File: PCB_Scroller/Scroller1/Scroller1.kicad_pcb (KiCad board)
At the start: 2 copper layers, 154.8 x 94.6 mm, 66 parts

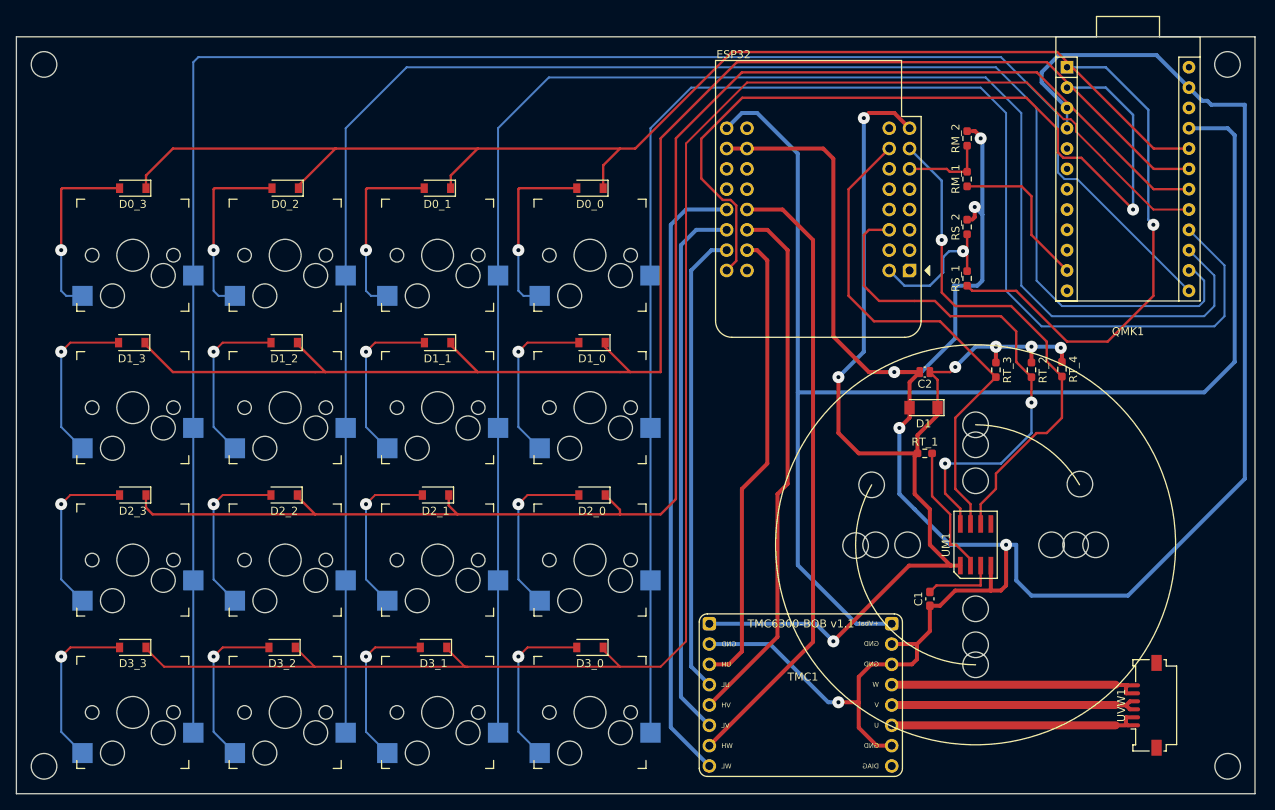
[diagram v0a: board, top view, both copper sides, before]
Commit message: Updates
Not sure if the ESP32 works...
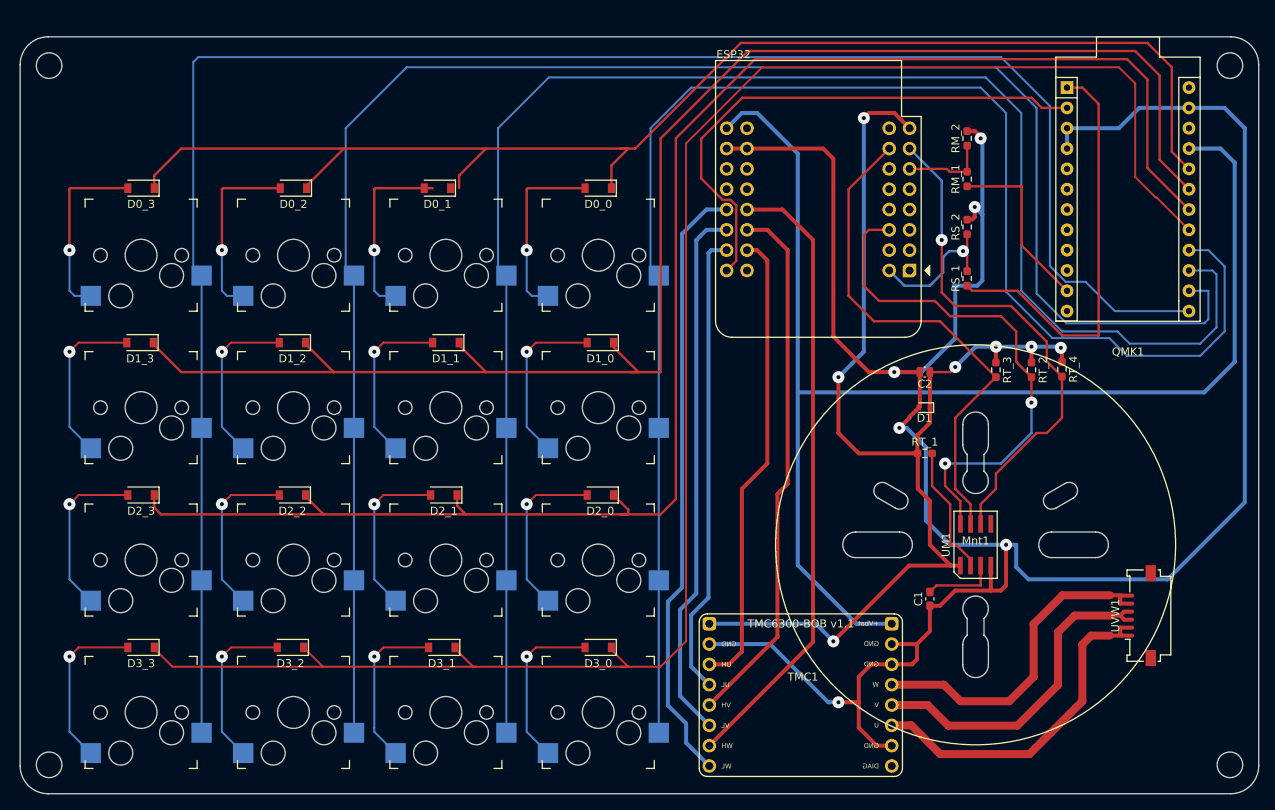
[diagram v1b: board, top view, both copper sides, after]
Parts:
- removed 2208_1, 2208_2, 2208_3, 2208_4, 3508_1, 3508_2, 3508_3, 3508_4, 6010_1, 6010_2, 6010_3, 6010_4, E6B2_1, E6B2_2: M3, MountingHole:MountingHole_3.2mm_M3
- added Mnt1: -, MT6701:BLDC Mount, F.Cu at (183.8, 117.1)
- D1: footprint Diode_SMD:D_MiniMELF -> Diode_SMD:D_SOD-523
- moved UVW1 11.2 mm to (203.9, 125.9)
- moved QMK1 2.54 mm to (210.4, 87.9)
- moved D0_0 1.04 mm to (136.6, 72.5)
- moved D0_2 1.04 mm to (98.5, 72.5)
- moved D1_0 1.04 mm to (136.8, 91.8)
- moved D1_2 1.04 mm to (98.4, 91.8)
- moved D1_3 1.04 mm to (79.3, 91.8)
- moved D2_0 1.04 mm to (136.8, 110.9)
- moved D2_2 1.04 mm to (98.4, 110.9)
- moved D3_0 1.04 mm to (136.6, 129.9)
- moved D3_1 1.04 mm to (117.0, 129.9)
- moved D3_2 1.04 mm to (98.1, 129.9)
- moved SW_0_0 1.04 mm to (136.6, 80.9)
- moved SW_0_1 1.04 mm to (117.5, 80.9)
- moved SW_0_2 1.04 mm to (98.5, 80.9)
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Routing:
- net Net-(ESP32-Pad16): track 104.4 -> 67.7 mm, vias 1 -> 0
- net GND: track 320.2 -> 306.7 mm
- net Net-(QMK1-Pad1): track 64.4 -> 52.8 mm, vias 1 -> 0
- net /U_Out: track 33.2 -> 44.3 mm
- net /V_Out: track 32.8 -> 42.7 mm
- net /W_Out: track 33.2 -> 42.7 mm
- net /Row 4: track 215.7 -> 224.6 mm
- net /Row 3: track 197.0 -> 205.9 mm
- net /Col 4: track 224.9 -> 233.4 mm
- net /Row 2: track 186.0 -> 194.4 mm
- net /Row 1: track 162.4 -> 170.6 mm
- net /Col 2: track 201.6 -> 205.9 mm
- net /Col 3: track 216.3 -> 219.6 mm
- net /Col 1: track 188.0 -> 191.1 mm
- net +5V: track 168.6 -> 165.5 mm
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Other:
- outline, holes or cut-outs redrawn
